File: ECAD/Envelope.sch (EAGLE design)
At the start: 15 parts

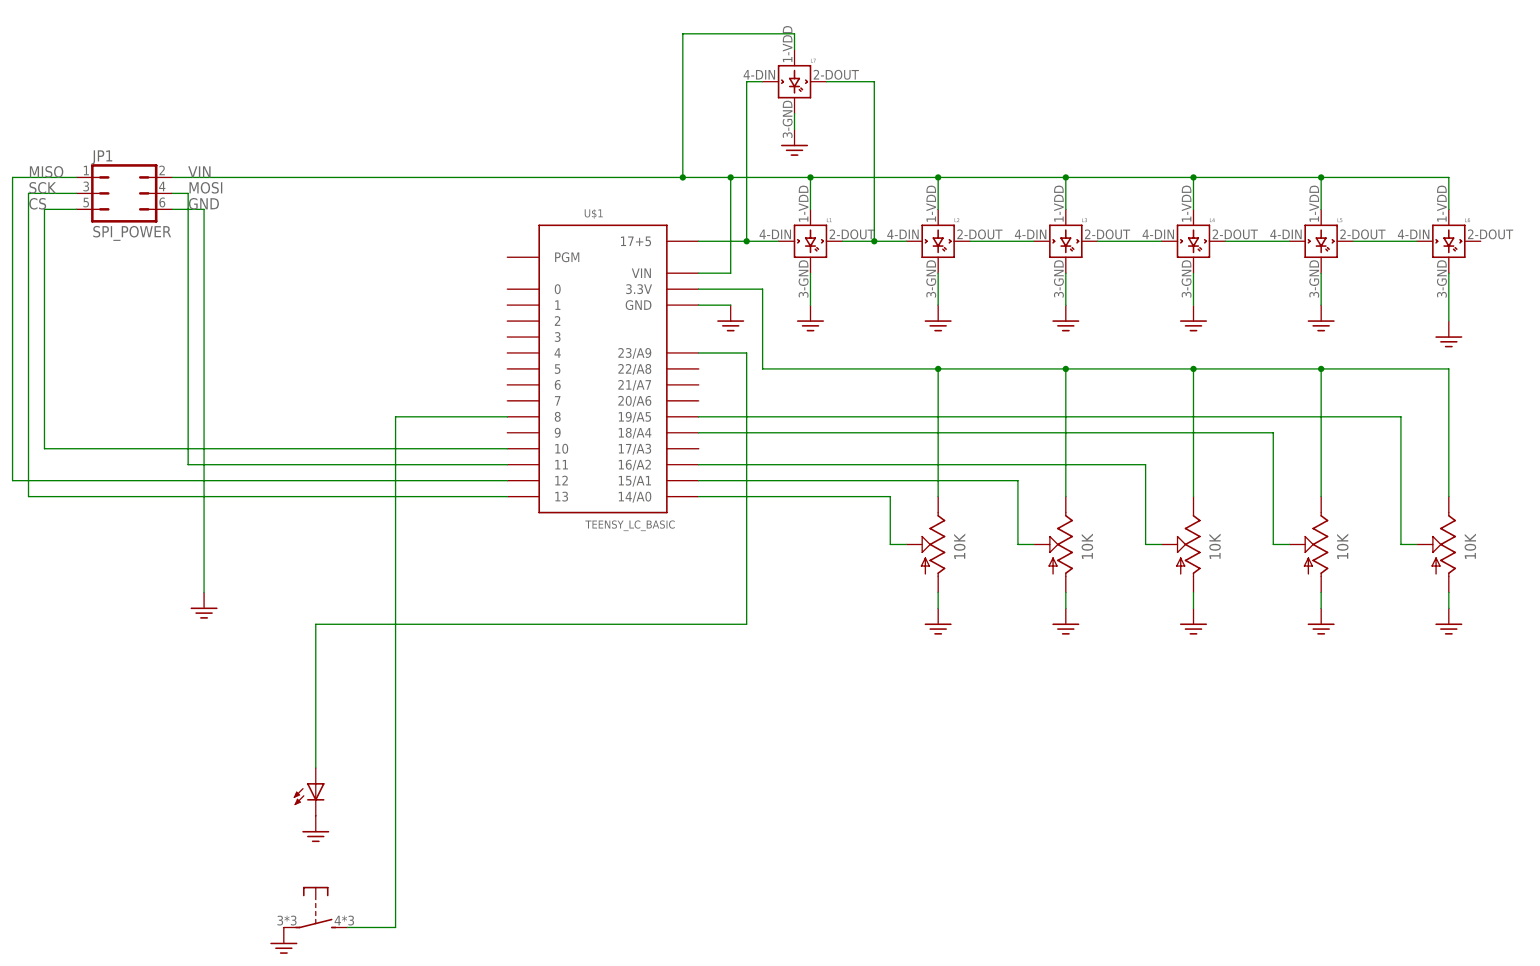
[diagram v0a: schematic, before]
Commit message: Designed the Envelope board.  Fairly straightforward, except that it has three variants.
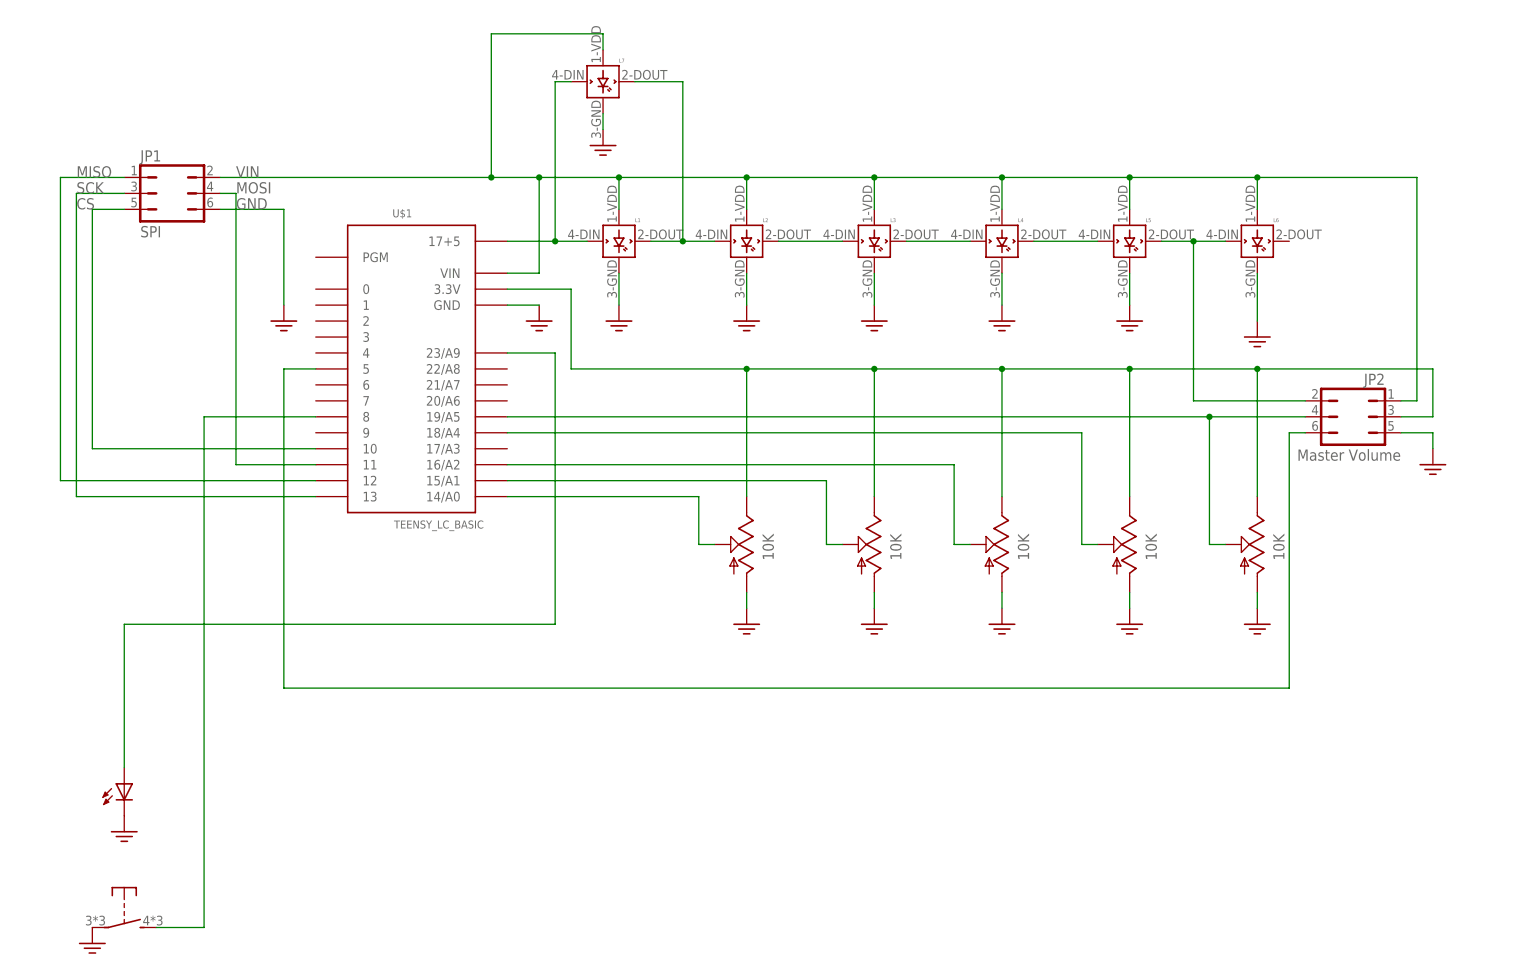
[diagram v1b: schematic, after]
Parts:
- added JP2: Master Volume, SynthLib:JP3Q
- JP1: value SPI_POWER -> SPI
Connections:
- new net N$12: JP2.6, U$1.5
- net 3.3V: now also JP2.3
- net GND: now also JP2.5
- net N$26: now also JP2.2
- net N$27: now also JP2.4
- net VIN: now also JP2.1
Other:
- moved on the sheet: JP1, L1, L2, L3, L4, L5, L6, L7, U$1
